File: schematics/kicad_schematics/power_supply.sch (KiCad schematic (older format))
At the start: 28 parts, among them Q3 MOSFET_N, Q4 NMOS, U10 LTC3827, U11 LTC1771

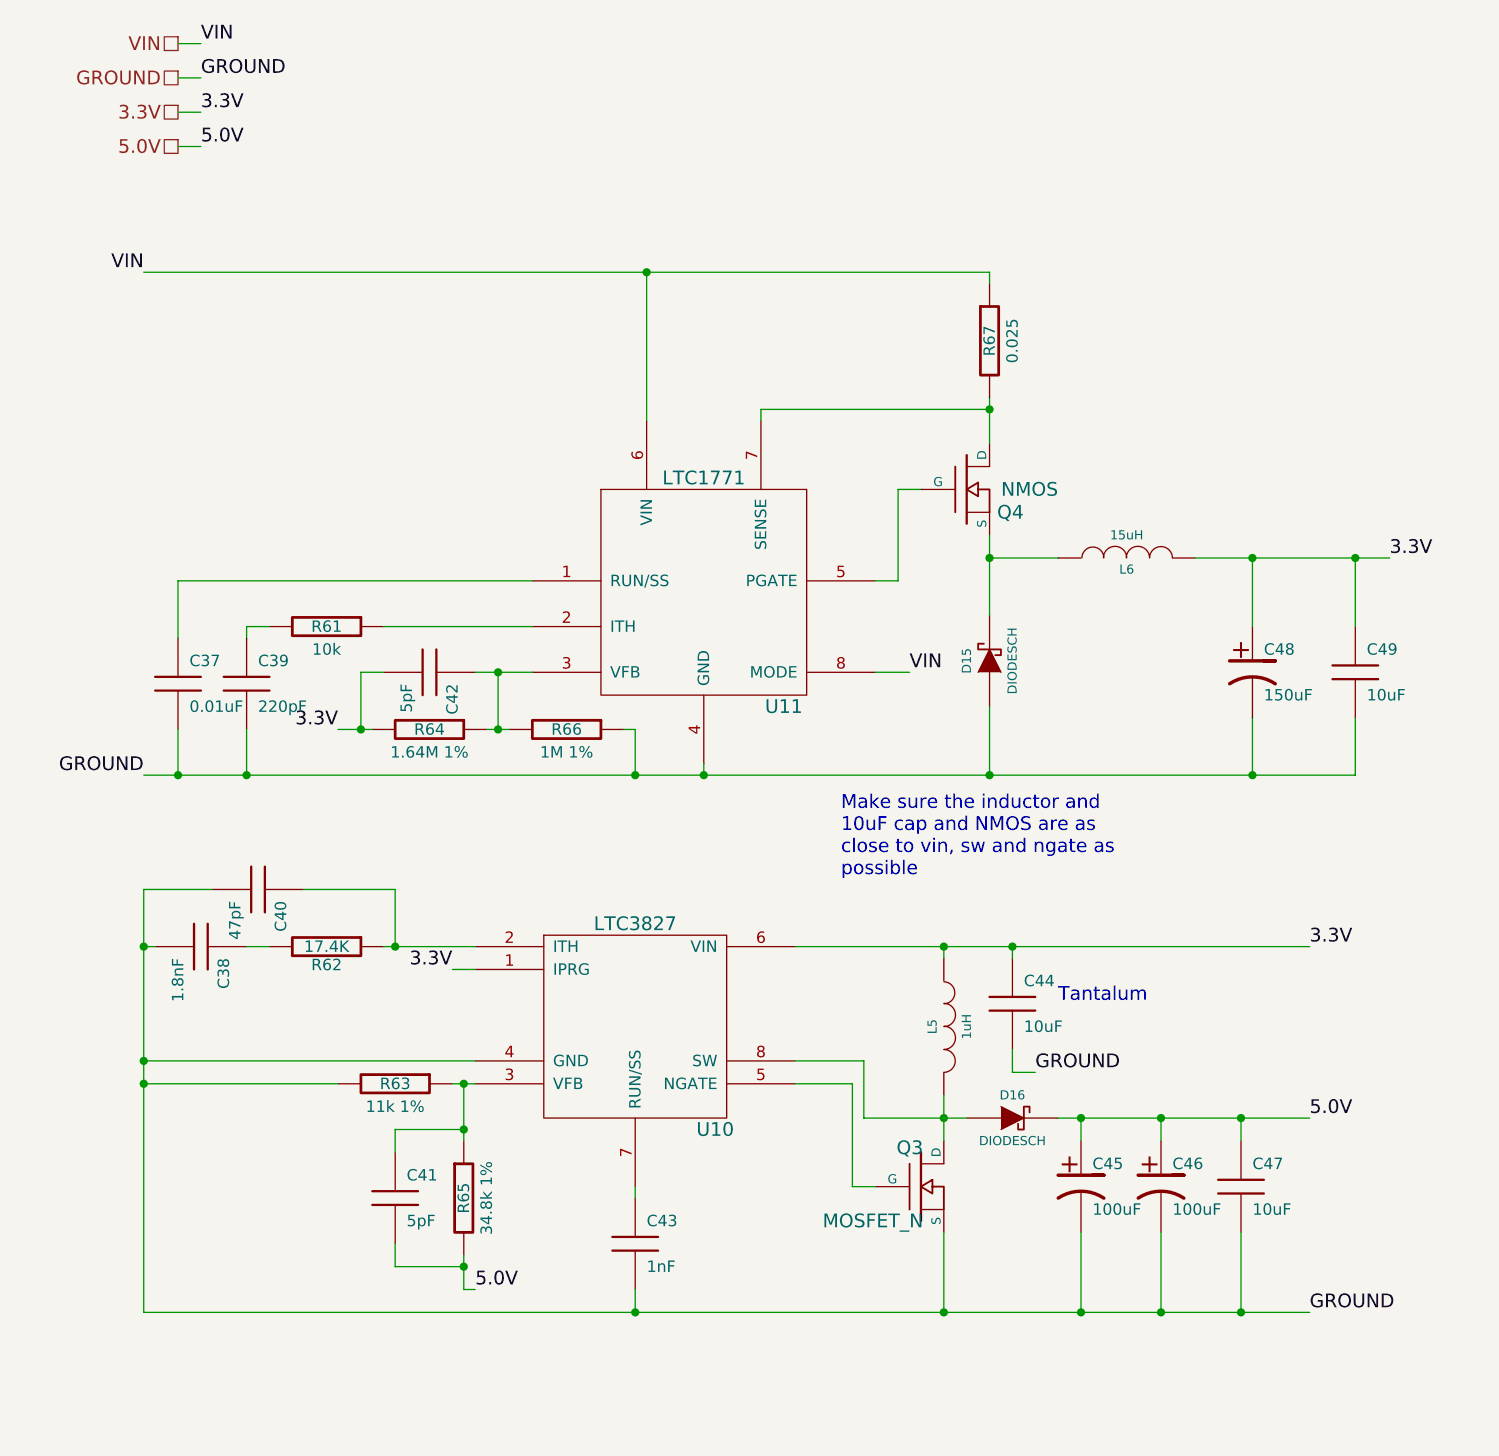
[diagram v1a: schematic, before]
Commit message: Fixed some data modules
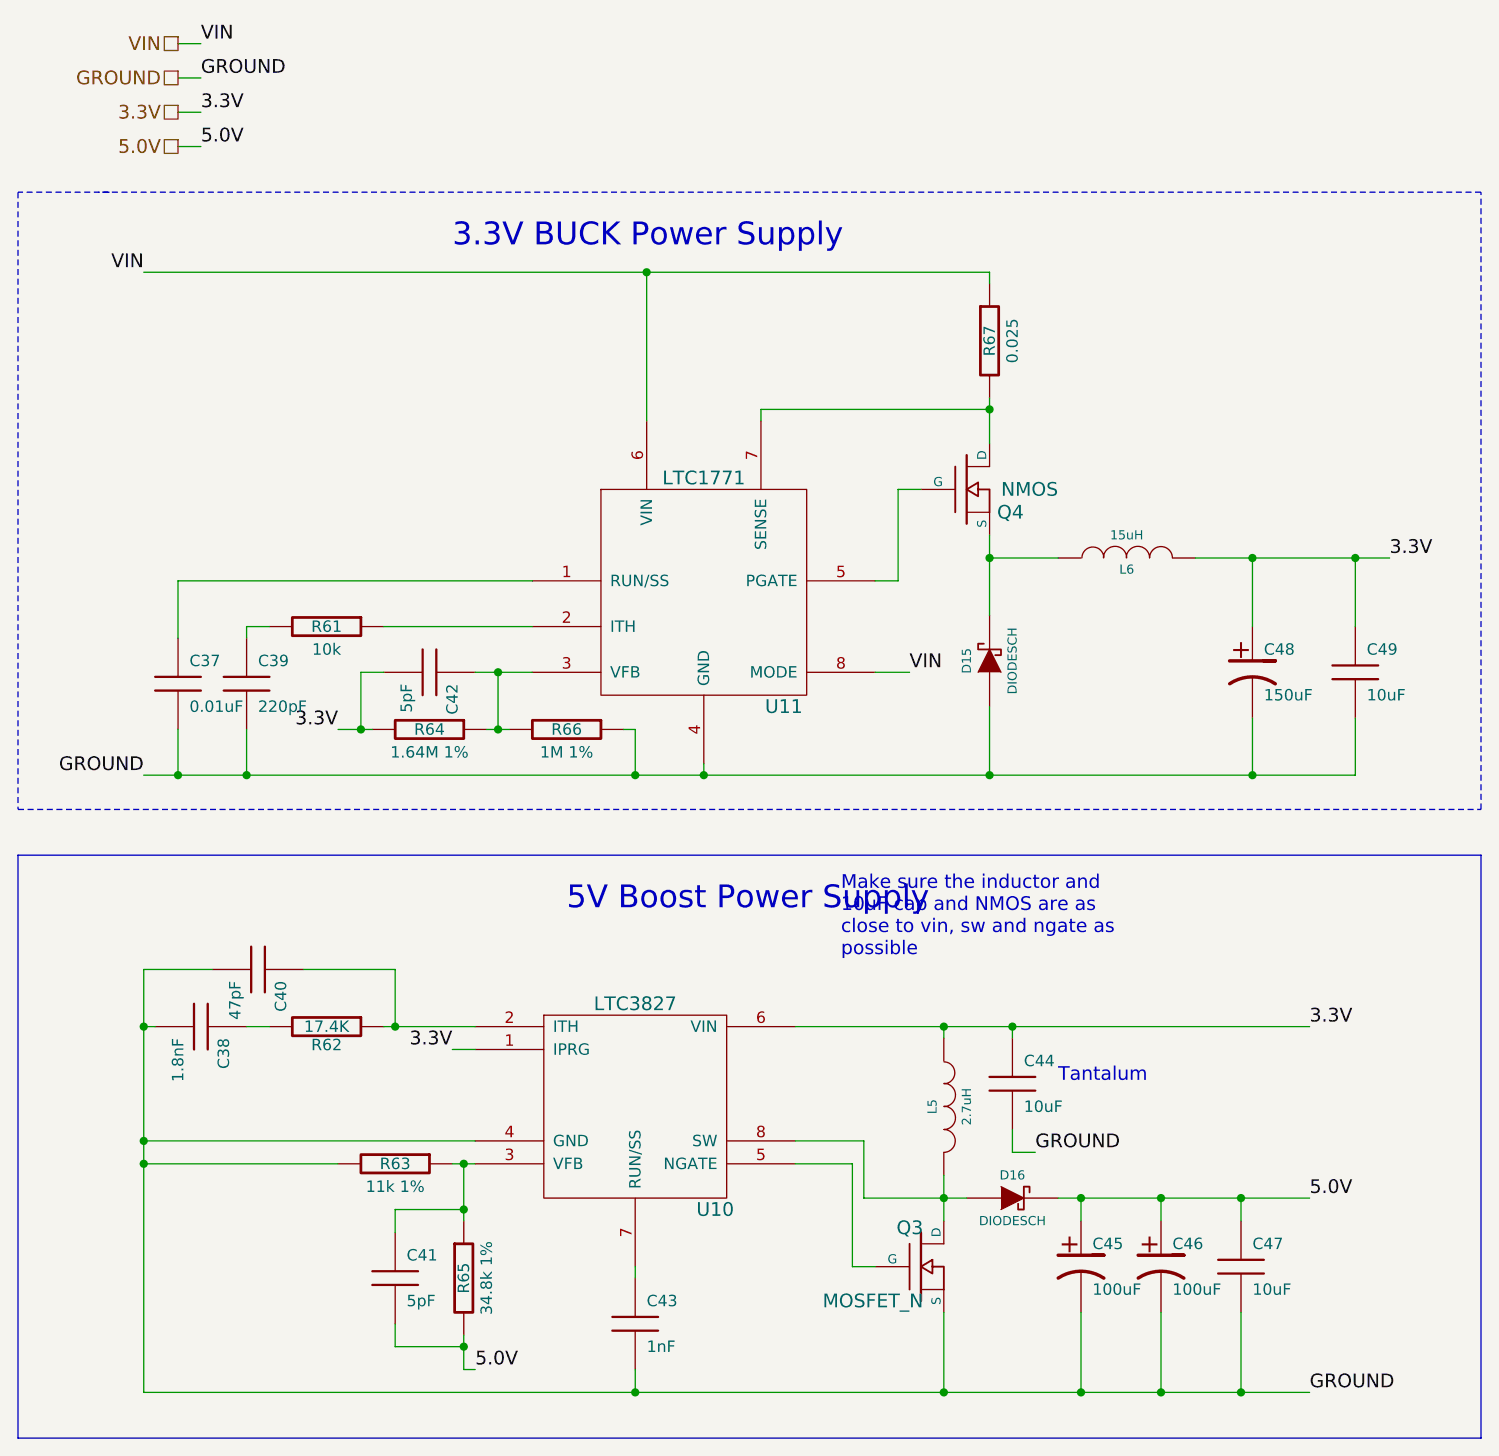
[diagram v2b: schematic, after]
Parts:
- L5: value 1uH -> 2.7uH
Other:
- note added: "3.3V BUCK Power Supply"
- note added: "5V Boost Power Supply"
- moved on the sheet: C38, C40, C41, C43, C44, C45, C46, C47, D16, L5, Q3, R62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

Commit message: added npn datasheet
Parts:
- D15, D16: footprint (none) -> SC-59
- L5: footprint (none) -> SD6030-Inductor
- L6: footprint (none) -> DR125-Inductors
- Q3: footprint (none) -> SSOT6_Mosfet-1256Connected
- Q4: footprint (none) -> -SO-08
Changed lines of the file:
@@
-EESchema Schematic File Version 2  date Sat 13 Mar 2010 03:45:55 PM EST
+EESchema Schematic File Version 2  date Sat 13 Mar 2010 04:13:45 PM EST
 LIBS:power
 LIBS:device
@@
 F 0 "D16" H 5950 5900 40  0000 C CNN
 F 1 "DIODESCH" H 5950 5700 40  0000 C CNN
+F 2 "SC-59" H 5950 5800 60  0001 C CNN
 	1    5950 5800
 	1    0    0    -1
@@
 F 0 "L5" V 5600 5400 40  0000 C CNN
 F 1 "2.7uH" V 5750 5400 40  0000 C CNN
+F 2 "SD6030-Inductor" H 5650 5400 60  0001 C CNN
 	1    5650 5400
 	1    0    0    -1
@@
 F 0 "Q3" H 5560 6270 60  0000 R CNN
 F 1 "MOSFET_N" H 5560 5950 60  0000 R CNN
+F 2 "SSOT6_Mosfet-1256Connected" H 5550 6100 60  0001 C CNN
 	1    5550 6100
 	1    0    0    -1
@@
 F 0 "L6" V 6400 3000 40  0000 C CNN
 F 1 "15uH" V 6550 3000 40  0000 C CNN
+F 2 "DR125-Inductors" H 6450 3000 60  0001 C CNN
 	1    6450 3000
 	0    -1   -1   0
@@
 F 0 "D15" H 5850 3550 40  0000 C CNN
 F 1 "DIODESCH" H 5850 3350 40  0000 C CNN
+F 2 "SC-59" H 5850 3450 60  0001 C CNN
 	1    5850 3450
 	0    -1   -1   0
@@
 F 0 "Q4" H 6000 2600 60  0000 R CNN
 F 1 "NMOS" H 6150 2700 60  0000 R CNN
+F 2 "-SO-08" H 5750 2700 60  0001 C CNN
 	1    5750 2700
 	1    0    0    -1
